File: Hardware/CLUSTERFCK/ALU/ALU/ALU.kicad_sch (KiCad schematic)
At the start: 33 parts, among them J1 Conn_02x08_Counter_Clockwise, J2 Conn_02x08_Counter_Clockwise, J3 Conn_02x08_Counter_Clockwise, U1 74LS86, U2 74LS283, U3 74LS283, U4 74LS86, U5 74LS02, U6 74LS08, U7 74LS245

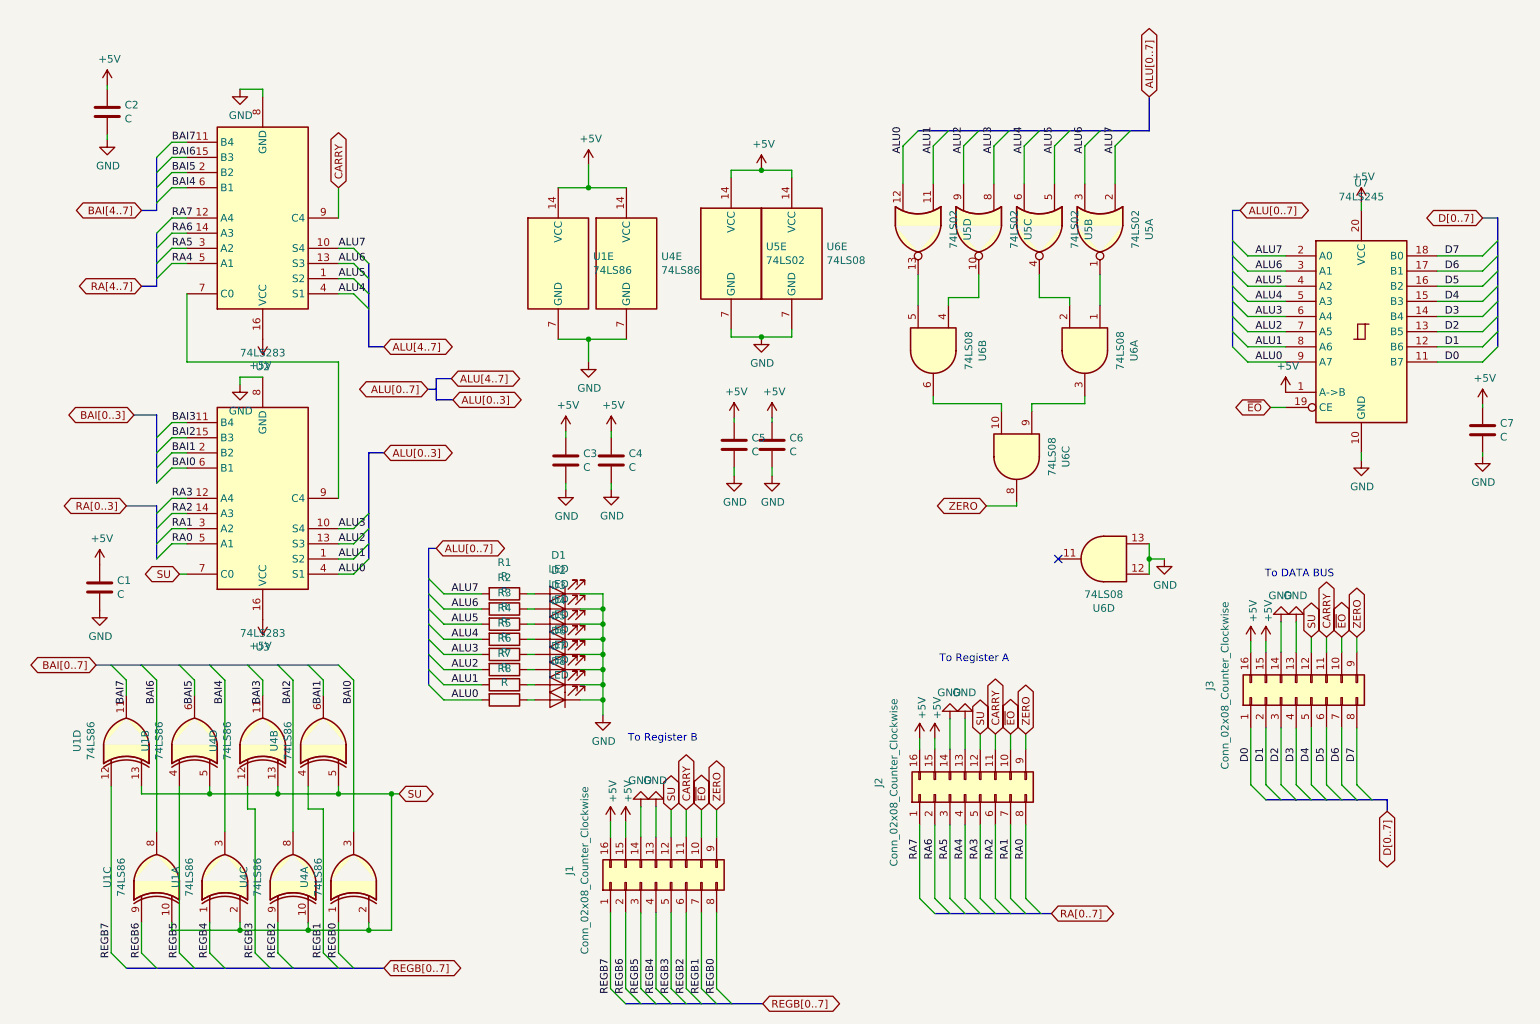
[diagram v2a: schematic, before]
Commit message: 0046|6|Alu Module
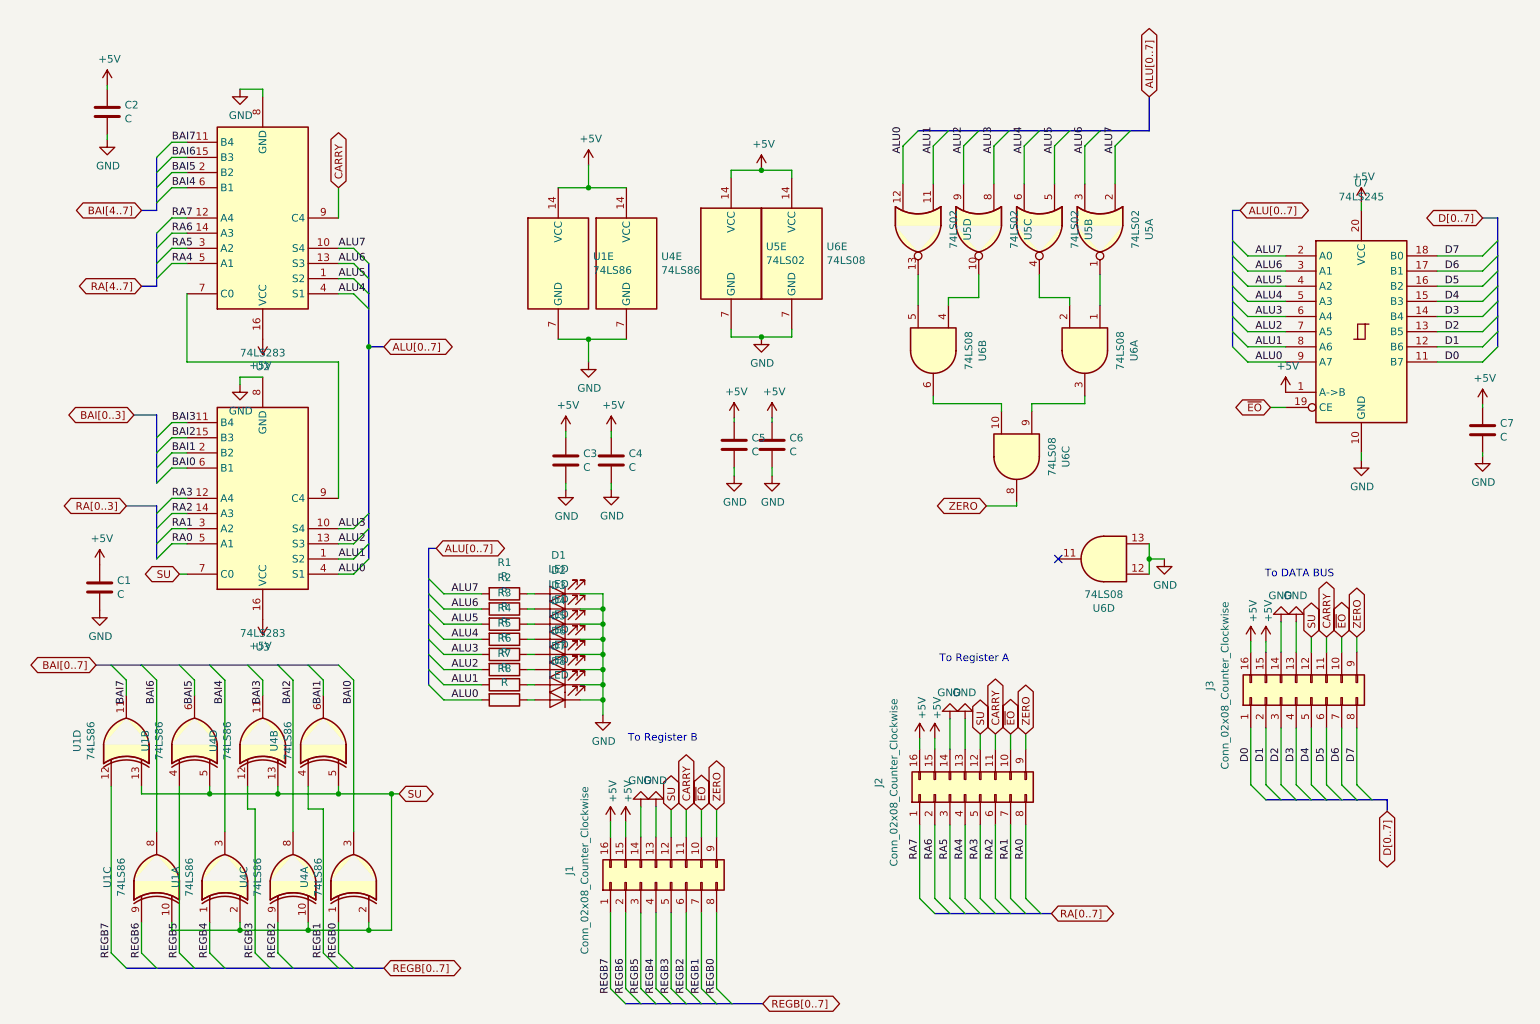
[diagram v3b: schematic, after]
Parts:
- J1, J2, J3: footprint (none) -> Connector_PinHeader_2.54mm:PinHeader_2x08_P2.54mm_Horizontal
- U2, U3: footprint Package_SO:SOIC-16W_5.3x10.2mm_P1.27mm -> Package_SO:SO-16_5.3x10.2mm_P1.27mm
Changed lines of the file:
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@@
   (junction (at 148.3614 63.119) (diameter 0) (color 0 0 0 0))
   (junction (at 213.36 100.33) (diameter 0) (color 0 0 0 0))
+  (junction (at 82.55 64.77) (diameter 0) (color 0 0 0 0))
   (no_connect (at 198.12 100.33))
   (bus_entry (at 39.37 118.11) (size 2.54 2.54)
@@
     (stroke (width 0) (type solid) (color 0 0 0 0))
   )
-  (bus (pts (xy 46.99 33.02) (xy 46.99 35.56))
-    (stroke (width 0) (type solid) (color 0 0 0 0))
-  )
-  (bus (pts (xy 46.99 35.56) (xy 46.99 40.64))
-    (stroke (width 0) (type solid) (color 0 0 0 0))
-  )
-  (bus (pts (xy 46.99 40.64) (xy 46.99 41.91))
-    (stroke (width 0) (type solid) (color 0 0 0 0))
-  )
-  (bus (pts (xy 46.99 45.72) (xy 46.99 50.8))
-    (stroke (width 0) (type solid) (color 0 0 0 0))
-  )
-  (bus (pts (xy 46.99 50.8) (xy 46.99 54.61))
+  (bus (pts (xy 46.99 33.02) (xy 46.99 38.1))
+    (stroke (width 0) (type solid) (color 0 0 0 0))
+  )
+  (bus (pts (xy 46.99 38.1) (xy 46.99 41.91))
+    (stroke (width 0) (type solid) (color 0 0 0 0))
+  )
+  (bus (pts (xy 46.99 45.72) (xy 46.99 48.26))
+    (stroke (width 0) (type solid) (color 0 0 0 0))
+  )
+  (bus (pts (xy 46.99 48.26) (xy 46.99 53.34))
+    (stroke (width 0) (type solid) (color 0 0 0 0))
+  )
+  (bus (pts (xy 46.99 53.34) (xy 46.99 54.61))
     (stroke (width 0) (type solid) (color 0 0 0 0))
   )
@@
     (stroke (width 0) (type solid) (color 0 0 0 0))
   )
-  (bus (pts (xy 66.04 168.91) (xy 69.85 168.91))
+  (bus (pts (xy 66.04 168.91) (xy 77.47 168.91))
     (stroke (width 0) (type solid) (color 0 0 0 0))
   )
@@
     (stroke (width 0) (type solid) (color 0 0 0 0))
   )
-  (bus (pts (xy 69.85 168.91) (xy 80.01 168.91))
-    (stroke (width 0) (type solid) (color 0 0 0 0))
-  )
-  (bus (pts (xy 80.01 168.91) (xy 85.09 168.91))
+  (bus (pts (xy 77.47 168.91) (xy 85.09 168.91))
     (stroke (width 0) (type solid) (color 0 0 0 0))
   )
@@
     (stroke (width 0) (type solid) (color 0 0 0 0))
   )
-  (bus (pts (xy 82.55 82.55) (xy 82.55 92.71))
+  (bus (pts (xy 82.55 64.77) (xy 82.55 92.71))
     (stroke (width 0) (type solid) (color 0 0 0 0))
   )
@@
     (stroke (width 0) (type solid) (color 0 0 0 0))
   )
-  (bus (pts (xy 85.09 82.55) (xy 82.55 82.55))
-    (stroke (width 0) (type solid) (color 0 0 0 0))
-  )
-  (bus (pts (xy 92.456 71.882) (xy 93.726 71.882))
-    (stroke (width 0) (type solid) (color 0 0 0 0))
-  )
-  (bus (pts (xy 92.583 98.552) (xy 92.583 103.632))
-    (stroke (width 0) (type solid) (color 0 0 0 0))
-  )
-  (bus (pts (xy 92.583 103.632) (xy 92.583 108.712))
-    (stroke (width 0) (type solid) (color 0 0 0 0))
-  )
-  (bus (pts (xy 92.583 108.712) (xy 92.583 113.792))
-    (stroke (width 0) (type solid) (color 0 0 0 0))
-  )
-  (bus (pts (xy 92.583 113.792) (xy 92.583 116.332))
-    (stroke (width 0) (type solid) (color 0 0 0 0))
-  )
-  (bus (pts (xy 92.583 116.332) (xy 92.583 121.412))
-    (stroke (width 0) (type solid) (color 0 0 0 0))
-  )
-  (bus (pts (xy 93.853 70.104) (xy 93.853 73.66))
-    (stroke (width 0) (type solid) (color 0 0 0 0))
-  )
-  (bus (pts (xy 93.853 73.66) (xy 96.647 73.66))
+  (bus (pts (xy 92.583 98.552) (xy 92.583 106.172))
+    (stroke (width 0) (type solid) (color 0 0 0 0))
+  )
+  (bus (pts (xy 92.583 106.172) (xy 92.583 111.252))
+    (stroke (width 0) (type solid) (color 0 0 0 0))
+  )
+  (bus (pts (xy 92.583 111.252) (xy 92.583 113.792))
+    (stroke (width 0) (type solid) (color 0 0 0 0))
+  )
+  (bus (pts (xy 92.583 113.792) (xy 92.583 118.872))
+    (stroke (width 0) (type solid) (color 0 0 0 0))
+  )
+  (bus (pts (xy 92.583 118.872) (xy 92.583 121.412))
     (stroke (width 0) (type solid) (color 0 0 0 0))
   )
@@
     (stroke (width 0) (type solid) (color 0 0 0 0))
   )
-  (bus (pts (xy 96.393 70.104) (xy 93.853 70.104))
-    (stroke (width 0) (type solid) (color 0 0 0 0))
-  )
   (bus (pts (xy 125.603 174.879) (xy 130.683 174.879))
     (stroke (width 0) (type solid) (color 0 0 0 0))
   )
-  (bus (pts (xy 130.683 174.879) (xy 133.223 174.879))
-    (stroke (width 0) (type solid) (color 0 0 0 0))
-  )
-  (bus (pts (xy 133.223 174.879) (xy 138.303 174.879))
-    (stroke (width 0) (type solid) (color 0 0 0 0))
-  )
-  (bus (pts (xy 138.303 174.879) (xy 143.383 174.879))
-    (stroke (width 0) (type solid) (color 0 0 0 0))
-  )
-  (bus (pts (xy 143.383 174.879) (xy 148.59 174.879))
+  (bus (pts (xy 130.683 174.879) (xy 135.763 174.879))
+    (stroke (width 0) (type solid) (color 0 0 0 0))
+  )
+  (bus (pts (xy 135.763 174.879) (xy 140.843 174.879))
+    (stroke (width 0) (type solid) (color 0 0 0 0))
+  )
+  (bus (pts (xy 140.843 174.879) (xy 148.59 174.879))
     (stroke (width 0) (type solid) (color 0 0 0 0))
   )
@@
     (stroke (width 0) (type solid) (color 0 0 0 0))
   )
-  (bus (pts (xy 271.78 49.53) (xy 271.78 52.07))
-    (stroke (width 0) (type solid) (color 0 0 0 0))
-  )
-  (bus (pts (xy 271.78 52.07) (xy 271.78 57.15))
+  (bus (pts (xy 271.78 49.53) (xy 271.78 54.61))
+    (stroke (width 0) (type solid) (color 0 0 0 0))
+  )
+  (bus (pts (xy 271.78 54.61) (xy 271.78 57.15))
     (stroke (width 0) (type solid) (color 0 0 0 0))
   )
@@
     (effects (font (size 1.27 1.27)) (justify left))
   )
-  (global_label "ALU[4..7]" (shape bidirectional) (at 85.09 64.77 0)
-    (effects (font (size 1.27 1.27)) (justify left))
-  )
-  (global_label "ALU[0..3]" (shape bidirectional) (at 85.09 82.55 0)
+  (global_label "ALU[0..7]" (shape bidirectional) (at 85.09 64.77 0)
     (effects (font (size 1.27 1.27)) (justify left))
   )
@@
     (effects (font (size 1.27 1.27)) (justify left))
   )
-  (global_label "ALU[0..7]" (shape bidirectional) (at 92.456 71.882 180)
-    (effects (font (size 1.27 1.27)) (justify right))
-  )
   (global_label "ALU[0..7]" (shape bidirectional) (at 93.853 98.552 0)
-    (effects (font (size 1.27 1.27)) (justify left))
-  )
-  (global_label "ALU[4..7]" (shape bidirectional) (at 96.393 70.104 0)
-    (effects (font (size 1.27 1.27)) (justify left))
-  )
-  (global_label "ALU[0..3]" (shape bidirectional) (at 96.647 73.66 0)
     (effects (font (size 1.27 1.27)) (justify left))
   )
@@
     (property "Reference" "J1" (id 0) (at 116.205 152.527 0))
     (property "Value" "Conn_02x08_Counter_Clockwise" (id 1) (at 118.745 152.527 0))
-    (property "Footprint" "" (id 2) (at 130.683 154.559 0)
+    (property "Footprint" "Connector_PinHeader_2.54mm:PinHeader_2x08_P2.54mm_Horizontal" (id 2) (at 130.683 154.559 0)
       (effects (font (size 1.27 1.27)) hide)
     )
@@
     (property "Reference" "J2" (id 0) (at 168.021 137.795 0))
     (property "Value" "Conn_02x08_Counter_Clockwise" (id 1) (at 170.561 137.795 0))
-    (property "Footprint" "" (id 2) (at 182.499 139.827 0)
+    (property "Footprint" "Connector_PinHeader_2.54mm:PinHeader_2x08_P2.54mm_Horizontal" (id 2) (at 182.499 139.827 0)
       (effects (font (size 1.27 1.27)) hide)
     )
@@
     (property "Reference" "J3" (id 0) (at 223.52 121.539 0))
     (property "Value" "Conn_02x08_Counter_Clockwise" (id 1) (at 226.06 121.539 0))
-    (property "Footprint" "" (id 2) (at 237.998 123.571 0)
+    (property "Footprint" "Connector_PinHeader_2.54mm:PinHeader_2x08_P2.54mm_Horizontal" (id 2) (at 237.998 123.571 0)
       (effects (font (size 1.27 1.27)) hide)
     )
@@
     (property "Reference" "U2" (id 0) (at 64.77 68.0974 0))
     (property "Value" "74LS283" (id 1) (at 64.77 65.786 0))
-    (property "Footprint" "Package_SO:SOIC-16W_5.3x10.2mm_P1.27mm" (id 2) (at 64.77 43.18 0)
+    (property "Footprint" "Package_SO:SO-16_5.3x10.2mm_P1.27mm" (id 2) (at 64.77 43.18 0)
       (effects (font (size 1.27 1.27)) hide)
     )
@@
     (property "Reference" "U3" (id 0) (at 64.77 115.0874 0))
     (property "Value" "74LS283" (id 1) (at 64.77 112.776 0))
-    (property "Footprint" "Package_SO:SOIC-16W_5.3x10.2mm_P1.27mm" (id 2) (at 64.77 90.17 0)
-      (effects (font (size 1.27 1.27)) hide)
-    )
+    (property "Footprint" "Package_SO:SO-16_5.3x10.2mm_P1.27mm" (id 2) (at 64.77 90.17 0)
+      (effects (font (size 1.27 1.27)) hide)
+    )
